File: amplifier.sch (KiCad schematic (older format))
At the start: 24 parts, among them J2 J_3.5mm_jack_SJ1-3523N, J3 J_2_screwterminal_2.54_282834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, Q1 Q_IRFZ44NPBF_N-Channel_Infine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, Q2 Q_IRFZ44NPBF_N-Channel_Infine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, U2 U_LM358AP_TI_DIP, U3 U_LM393N_NOPB, U4 U_TC4427M_Microchip

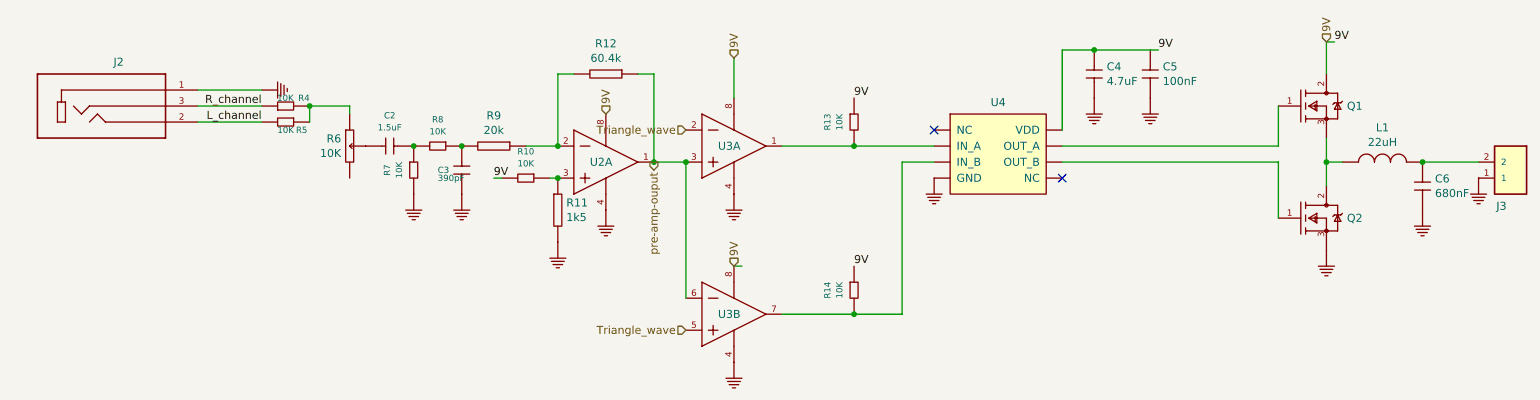
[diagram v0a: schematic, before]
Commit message: routed pcb
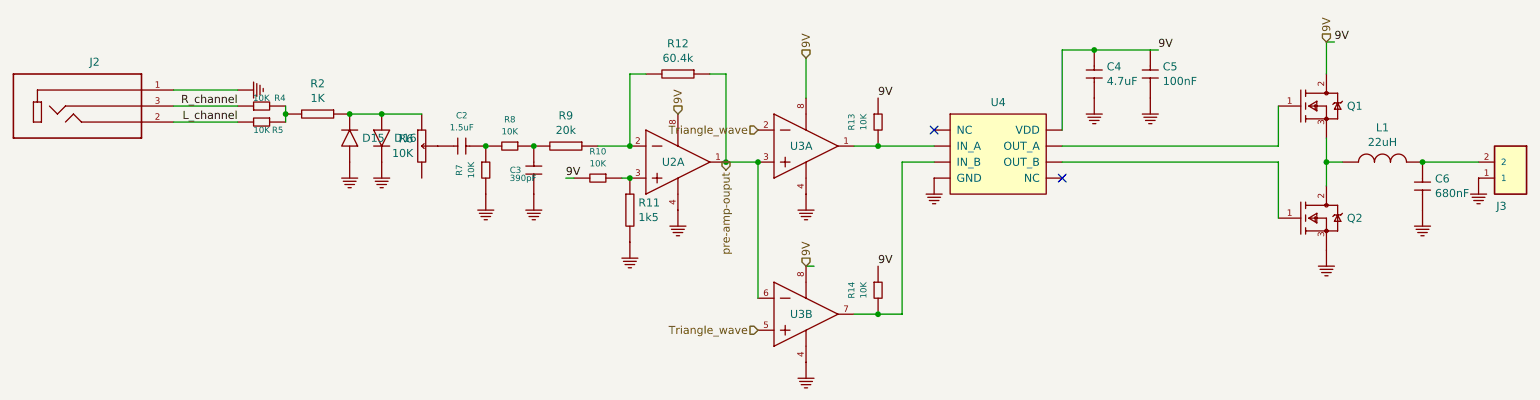
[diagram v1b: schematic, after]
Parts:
- added D15, D16: D_1N4148WS_SOD323F_ONSEMI, MAIN_PCB_LIB:D_1N4148_SOD-323F_ONSEMI, symbol Main_Library:D_1N4148WS_SOD323F_ONSEMI
- added R2: R_1K_0603, MAIN_PCB_LIB:R_0603, symbol Main_Library:R_1K_0603
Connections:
- net at R4.2, R5.1: now also R2.2; no longer R6.1
- new net: D15.C, D16.A, R2.1, R6.1
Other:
- moved on the sheet: C2, C3, J2, R10, R11, R12, R13, R14, R4, R5, R6, R7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
